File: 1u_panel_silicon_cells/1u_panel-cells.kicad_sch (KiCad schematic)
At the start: 33 parts, among them U13 LTC4411, U14 LTC4411, U15 LTC4411, U16 LTC4411, U5 LTC4411, U6 LTC4411, U8 LTC4411, U9 LTC4411

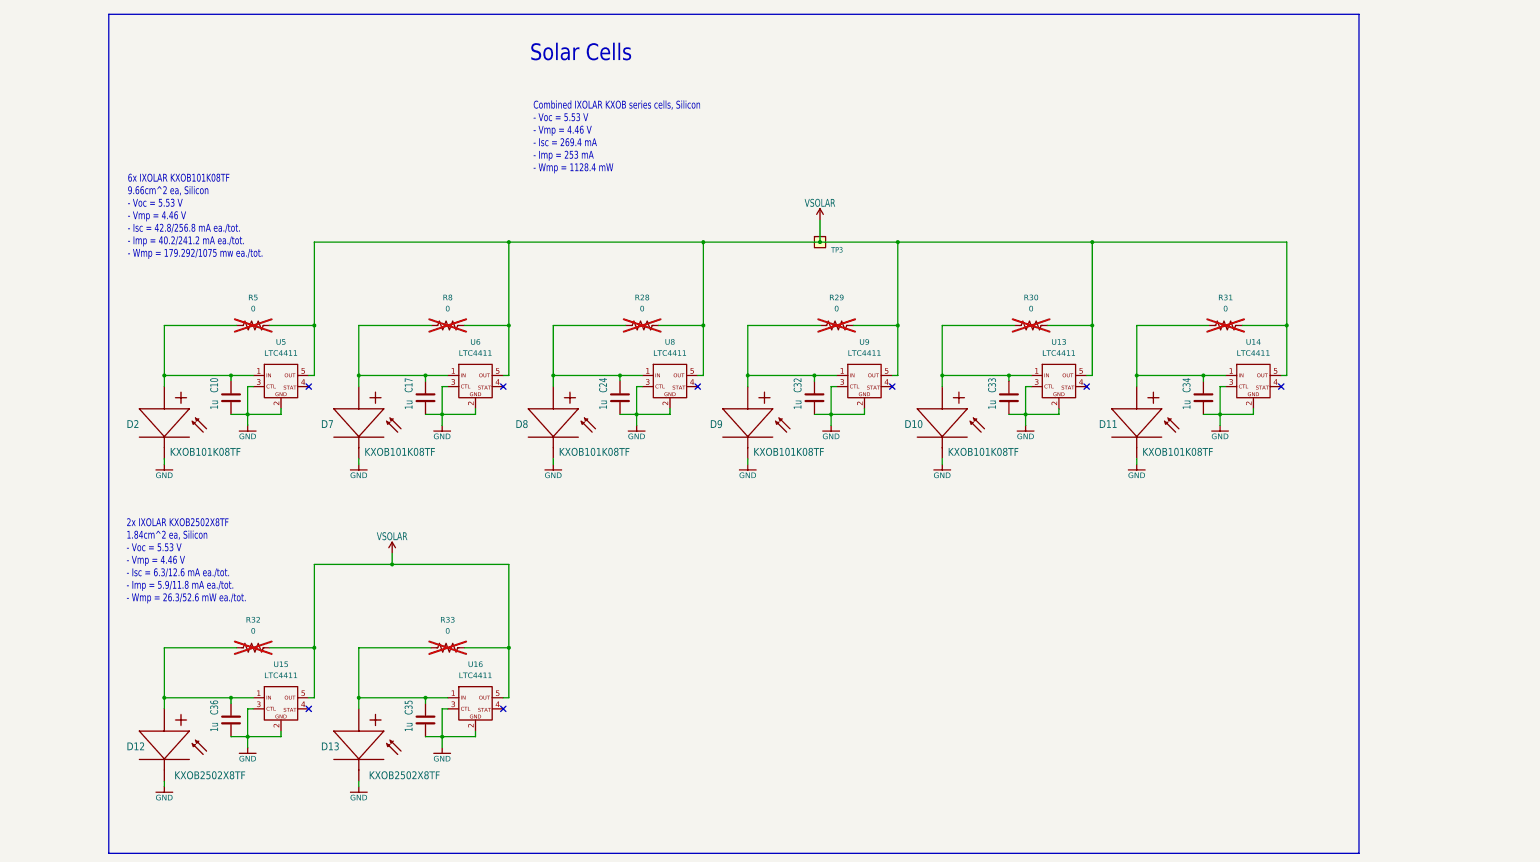
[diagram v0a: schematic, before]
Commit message: chages for https://github.com/oresat/oresat-solar-hardware/issues/53
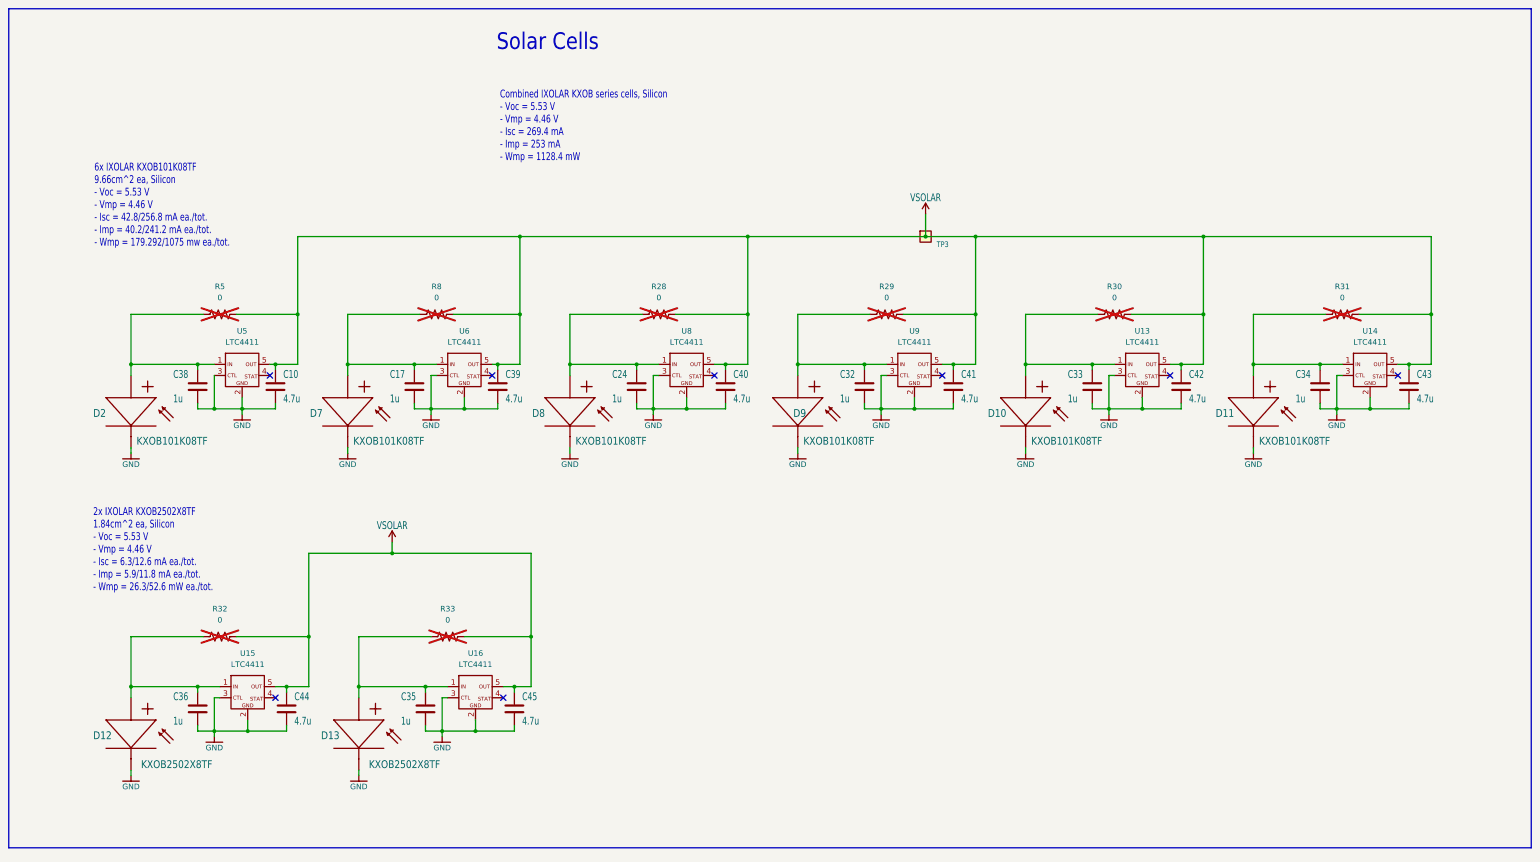
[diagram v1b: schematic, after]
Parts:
- added C38: 1u, oresat-passives:0603-C-NOSILK, symbol Device:C
- added C39, C40, C41, C42, C43, C44, C45: 4.7u, oresat-passives:0603-C-NOSILK, symbol Device:C
- C10: value 1u -> 4.7u; DPN 587-3473-1-ND -> 1276-1784-1-ND; MFR Taiyo Yuden -> Samsung Electro-Mechanics; MPN TMK107BJ105KAHT -> CL10A475KO8NNNC
- D12, D13: MPN KXOB25-02X8F-TR -> KXOB25-02X8TF-TR
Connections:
- net GND: now also C38.2, C39.2, C40.2, C41.2, C42.2, C43.2, C44.2, C45.2
- net VSOLAR: now also C10.1, C39.1, C40.1, C41.1, C42.1, C43.1, C44.1, C45.1
- net at D2.POS1 (A1), R5.1, U5.1: now also C38.1; no longer C10.1
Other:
- moved on the sheet: D10, D11, D12, D13, D2, D7, D8, D9, R28, R29, R30, R31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
